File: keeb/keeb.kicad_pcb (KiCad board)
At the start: 2 copper layers, 268 x 105 mm, 162 parts, among them J101 AVR-ISP-6, J102 USB_C_Receptacle_USB2.0, SW101 SW_Push, SW102 SW_Push, SW103 SW_Push, SW104 SW_Push, SW105 SW_Push, SW106 SW_Push, SW107 SW_Push, SW108 SW_Push, SW109 SW_Push, SW110 SW_Push, SW111 SW_Push, SW112 SW_Push, SW113 SW_Push, SW114 SW_Push, SW115 SW_Push, SW116 SW_Push, SW117 SW_Push, SW118 SW_Push, SW119 SW_Push, SW120 SW_Push, SW121 SW_Push, SW122 SW_Push, SW123 SW_Push, SW124 SW_Push, SW125 SW_Push, SW126 SW_Push, SW127 SW_Push, SW128 SW_Push, SW129 SW_Push, SW130 SW_Push, SW131 SW_Push, SW132 SW_Push, SW133 SW_Push, SW134 SW_Push, SW135 SW_Push, SW136 SW_Push, SW137 SW_Push, SW138 SW_Push, SW139 SW_Push, SW140 SW_Push, SW141 SW_Push, SW142 SW_Push, SW143 SW_Push, SW144 SW_Push, SW145 SW_Push, SW146 SW_Push, SW147 SW_Push, SW148 SW_Push, SW149 SW_Push, SW150 SW_Push, SW151 SW_Push, SW152 SW_Push, SW153 SW_Push, SW154 SW_Push, SW155 SW_Push, SW156 SW_Push, SW157 SW_Push, SW158 SW_Push, SW159 SW_Push, SW160 SW_Push, SW161 SW_Push, SW162 SW_Push, SW163 SW_Push, SW164 SW_Push, SW165 SW_Push, SW166 SW_Push, SW167 SW_Push, U101 TPD2S017, U102 ATmega32U4-MU, Y101 16Mhz

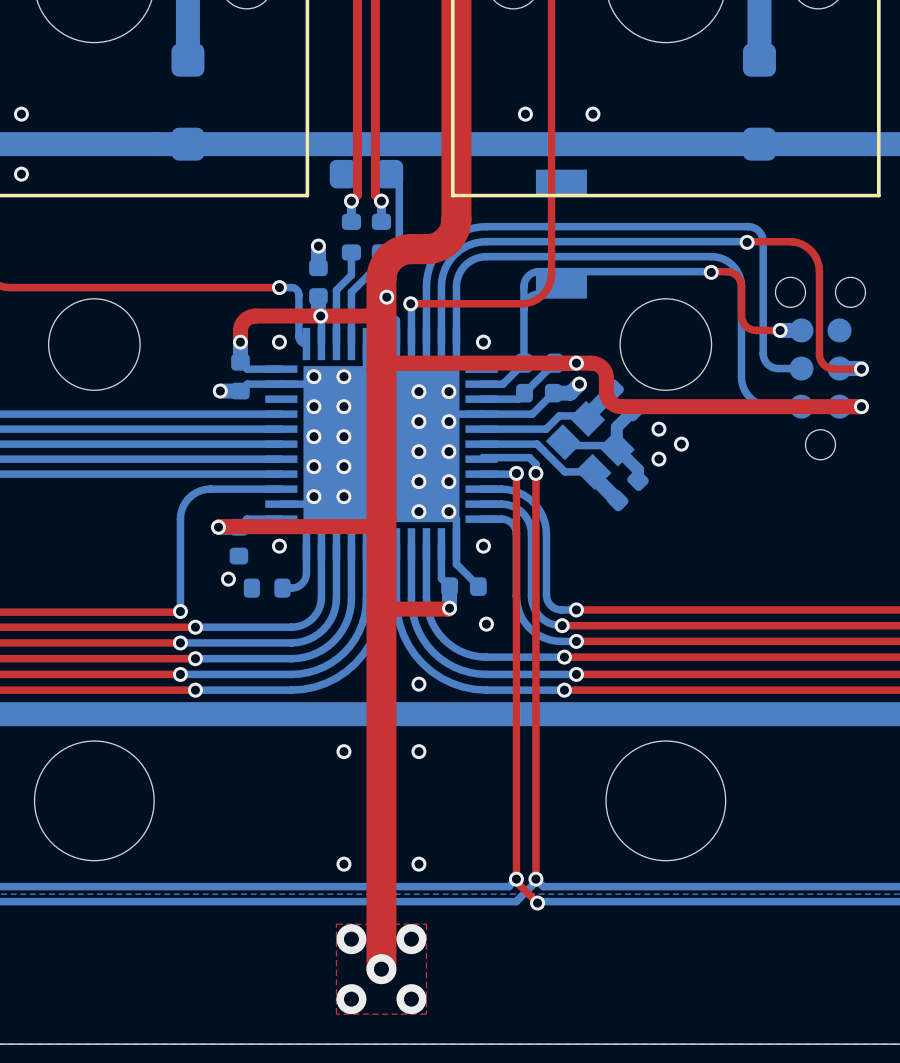
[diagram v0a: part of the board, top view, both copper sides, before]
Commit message: route cleanup
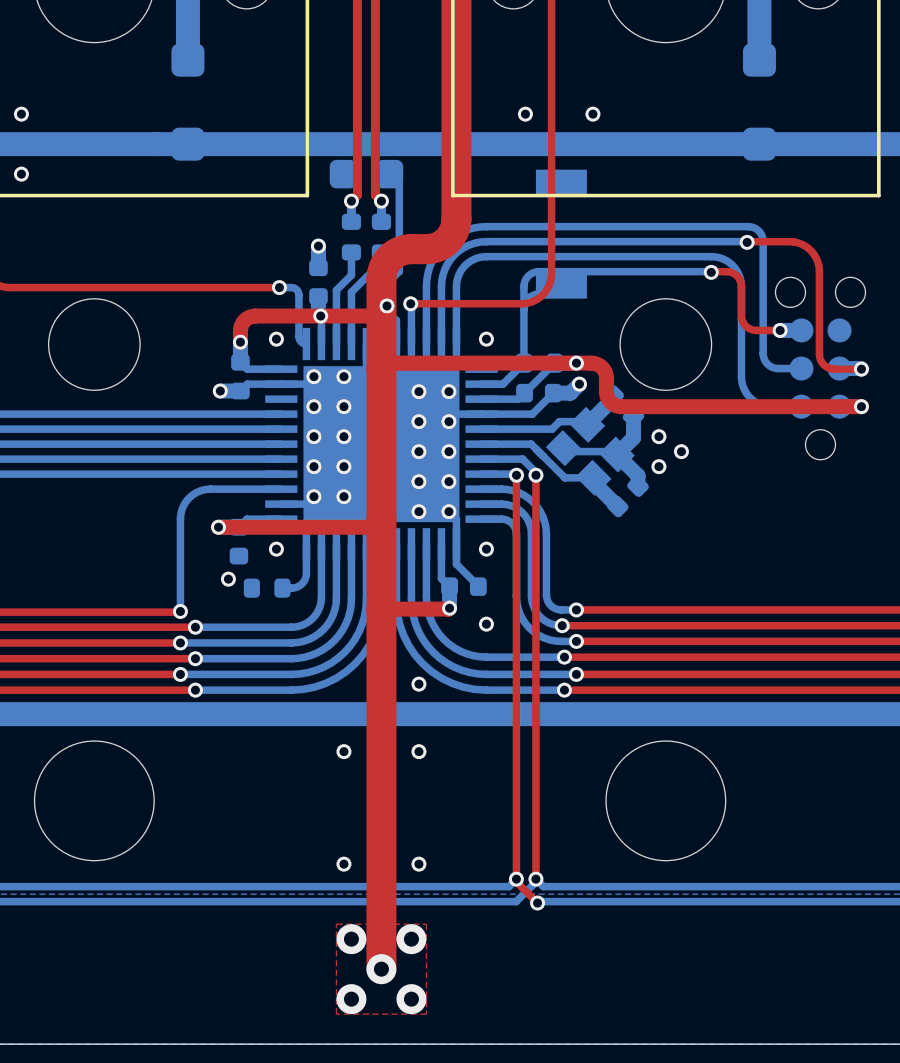
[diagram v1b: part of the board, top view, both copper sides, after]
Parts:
- moved C108 0.20 mm to (156.2, 111.7)
- moved C109 0.20 mm to (156.1, 108.7)
- moved Y101 0.20 mm to (155.0, 110.2)
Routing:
- net GND: track 43.8 -> 43.0 mm
